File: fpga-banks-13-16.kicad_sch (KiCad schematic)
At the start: 48 parts, among them U14 XC7A100T-FGG484, U15 Oscillator_100MHz_AMJMEFB

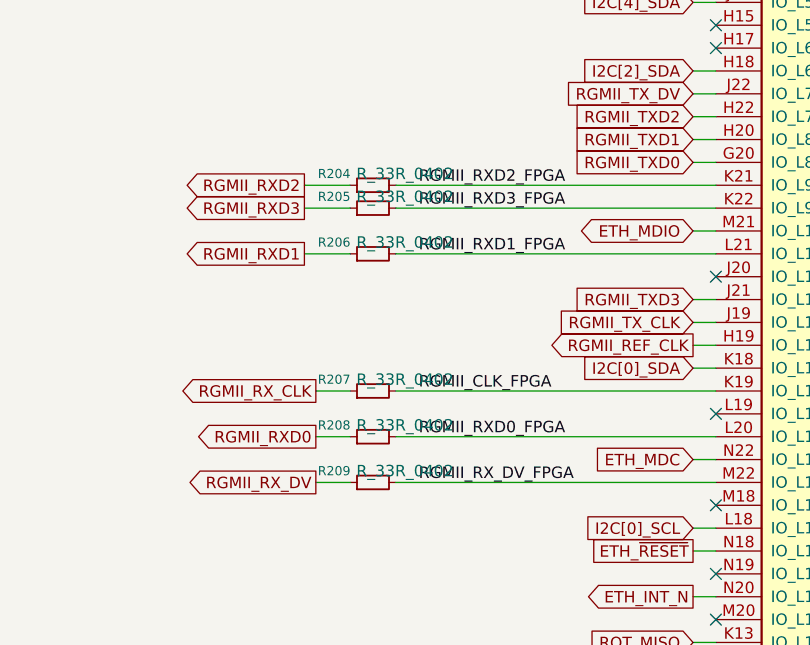
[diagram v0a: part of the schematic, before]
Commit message: version 1.0 complete
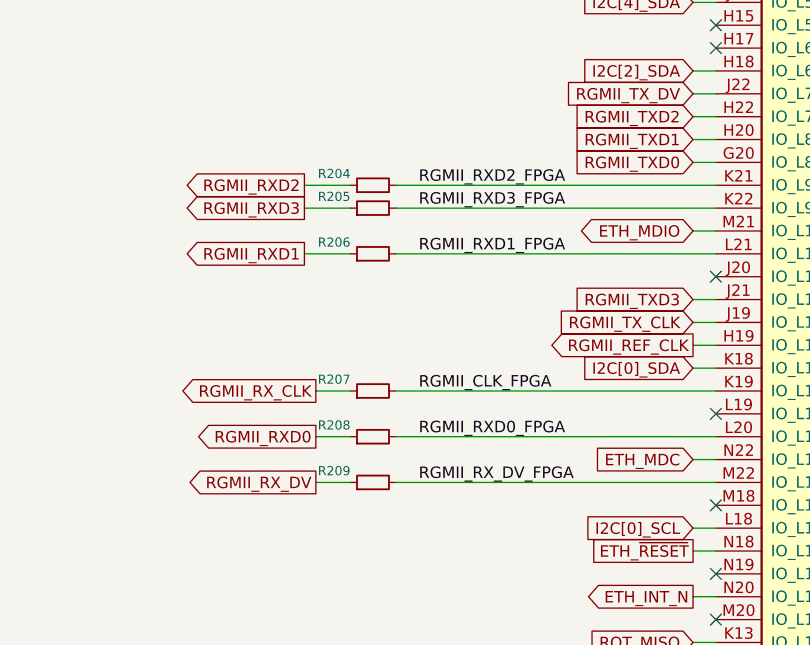
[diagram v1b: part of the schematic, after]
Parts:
- C92, C93, C94, C95: MPN C1210C476K8RACTU -> C1210C476K8RAC7210
- R133: MPN CR0402-FX-2201GLF -> AC0402FR-7D2K2L; Manufacturer Bourns -> YAGEO
- R134, R135: MPN CR0402-FX-4701GLF -> RC0402FR-7D4K7L; Manufacturer Bourns -> YAGEO
- R204, R205, R206, R207, R208, R209: MPN (none) -> MCS04020C3309FE000; Manufacturer (none) -> Vishay / Beyschlag
- U14: MPN XC7A100T-FGG484 -> XC7A100T-2FGG484C
- U15: MPN AMJMEFB-100.0000T -> ASEMB-100.000MHZ-XY-T

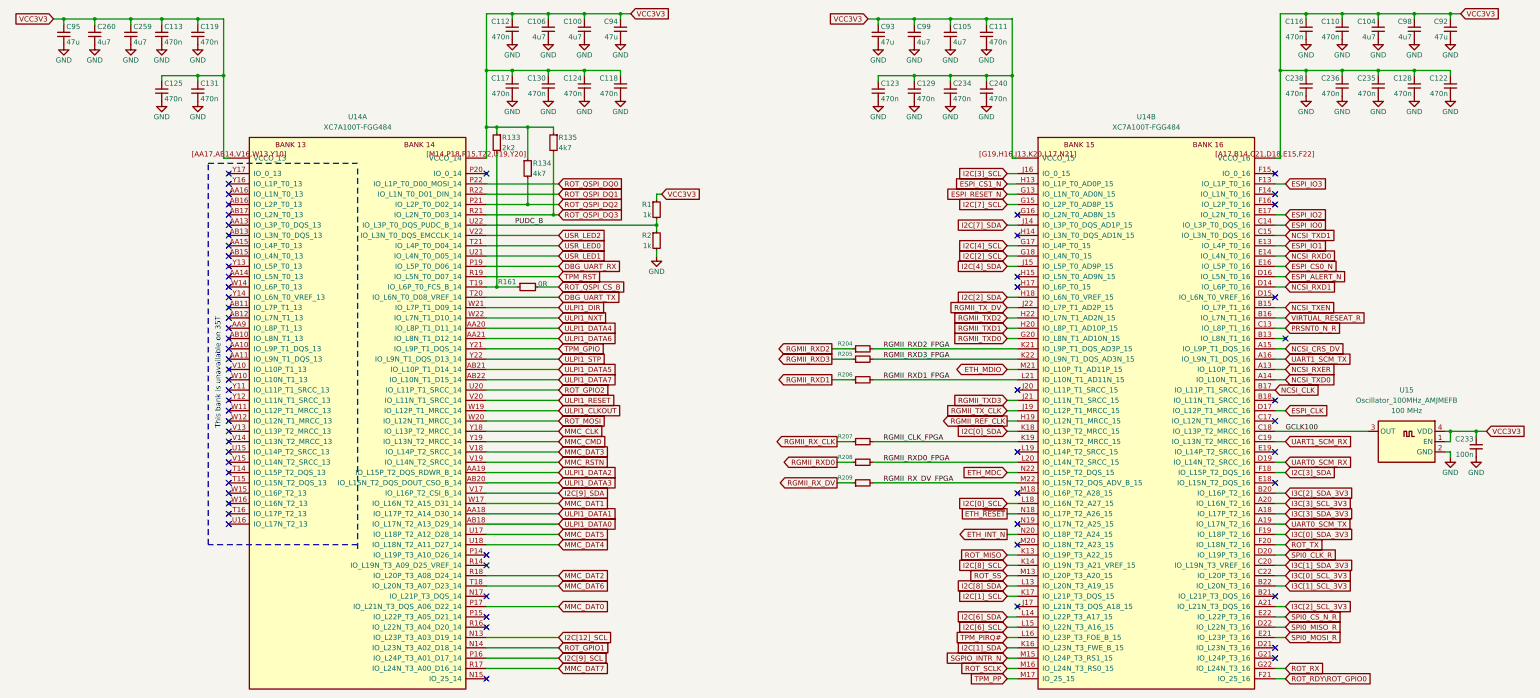
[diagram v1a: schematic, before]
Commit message: "In the process of upgrading the ddr memory"
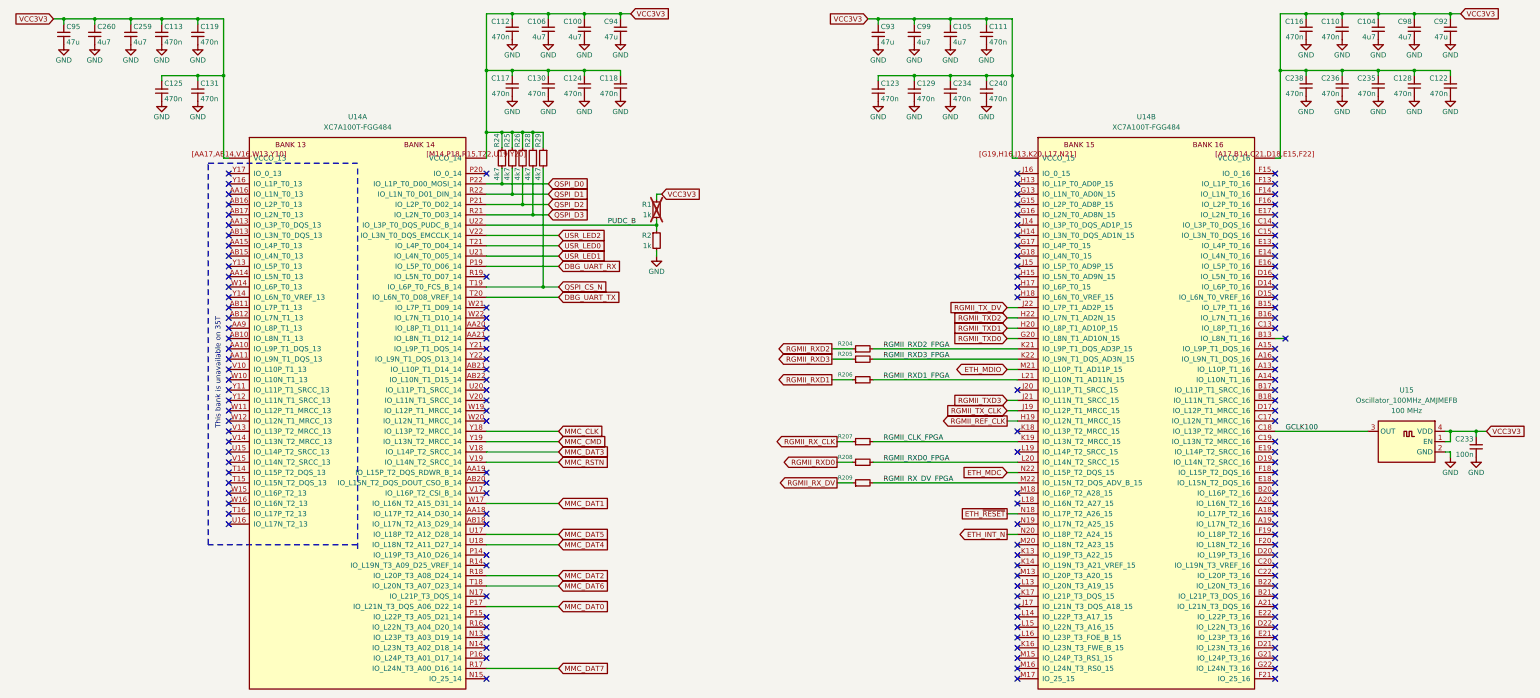
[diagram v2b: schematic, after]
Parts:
- removed R133: R_2k2_0402, antmicro-footprints:R_0402_1005Metric, symbol antmicroResistors0402:R_2k2_0402
- removed R134, R135: R_4k7_0402, antmicro-footprints:R_0402_1005Metric, symbol antmicroResistors0402:R_4k7_0402
- removed R161: R_0R_0402, antmicro-footprints:R_0402_1005Metric, symbol antmicroResistors0402:R_0R_0402
- added R24, R25, R26, R28, R29: R_4k7_0402, Resistor_SMD:R_0402_1005Metric, symbol antmicroResistors0402:R_4k7_0402
- C92, C93, C94, C95: footprint antmicro-footprints:C_1210_3225Metric -> Capacitor_SMD:C_1210_3225Metric
- R1: footprint antmicro-footprints:R_0402_1005Metric -> Resistor_SMD:R_0402_1005Metric; now not fitted; now left out of the parts list
- R2: footprint antmicro-footprints:R_0402_1005Metric -> Resistor_SMD:R_0402_1005Metric
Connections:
- net VCC3V3: now also R24.1, R25.1, R26.1, R28.1, R29.1
- net QSPI_CS_N: now reaches U14.T19 (IO_L6P_T0_FCS_B_14)
- net QSPI_CS_N: now also R29.2
- net ESPI_ALERT_N: no longer names the net of U14.D16 (IO_L5N_T0_16)
- net ESPI_CLK: no longer names the net of U14.D17 (IO_L12P_T1_MRCC_16)
- net ESPI_CS0_N: no longer names the net of U14.E16 (IO_L5P_T0_16)
- net ESPI_CS1_N: no longer names the net of U14.H13 (IO_L1P_T0_AD0P_15)
- net ESPI_IO0: no longer names the net of U14.C14 (IO_L3P_T0_DQS_16)
- net ESPI_IO1: no longer names the net of U14.E13 (IO_L4P_T0_16)
- net ESPI_IO2: no longer names the net of U14.E17 (IO_L2N_T0_16)
- net ESPI_IO3: no longer names the net of U14.F13 (IO_L1P_T0_16)
- net ESPI_RESET_N: no longer names the net of U14.G13 (IO_L1N_T0_AD0N_15)
- net I2C[0]_SCL: no longer names the net of U14.L18 (IO_L16N_T2_A27_15)
- net I2C[0]_SDA: no longer names the net of U14.K18 (IO_L13P_T2_MRCC_15)
- net I2C[12]_SCL: no longer names the net of U14.N13 (IO_L23P_T3_A03_D19_14)
- net I2C[1]_SCL: no longer names the net of U14.K17 (IO_L21P_T3_DQS_15)
- net I2C[1]_SDA: no longer names the net of U14.K16 (IO_L23N_T3_FWE_B_15)
- net I2C[2]_SCL: no longer names the net of U14.G18 (IO_L4N_T0_15)
- net I2C[2]_SDA: no longer names the net of U14.H18 (IO_L6N_T0_VREF_15)
- net I2C[3]_SCL: no longer names the net of U14.J16 (IO_0_15)
- net I2C[3]_SDA: no longer names the net of U14.F18 (IO_L15P_T2_DQS_16)
- net I2C[4]_SCL: no longer names the net of U14.G17 (IO_L4P_T0_15)
- net I2C[4]_SDA: no longer names the net of U14.J15 (IO_L5P_T0_AD9P_15)
- net I2C[6]_SCL: no longer names the net of U14.L15 (IO_L22N_T3_A16_15)
- net I2C[6]_SDA: no longer names the net of U14.L14 (IO_L22P_T3_A17_15)
- net I2C[7]_SCL: no longer names the net of U14.G15 (IO_L2P_T0_AD8P_15)
- net I2C[7]_SDA: no longer names the net of U14.J14 (IO_L3P_T0_DQS_AD1P_15)
- net I2C[8]_SCL: no longer names the net of U14.K14 (IO_L19N_T3_A21_VREF_15)
- net I2C[8]_SDA: no longer names the net of U14.L13 (IO_L20N_T3_A19_15)
- net I2C[9]_SCL: no longer names the net of U14.P16 (IO_L24P_T3_A01_D17_14)
- net I2C[9]_SDA: no longer names the net of U14.V17 (IO_L16P_T2_CSI_B_14)
- net I3C[0]_SCL_3V3: no longer names the net of U14.C22 (IO_L20P_T3_16)
- net I3C[0]_SDA_3V3: no longer names the net of U14.F19 (IO_L18P_T2_16)
- net I3C[1]_SCL_3V3: no longer names the net of U14.B22 (IO_L20N_T3_16)
- net I3C[1]_SDA_3V3: no longer names the net of U14.C20 (IO_L19N_T3_VREF_16)
- net I3C[2]_SCL_3V3: no longer names the net of U14.A21 (IO_L21N_T3_DQS_16)
- net I3C[2]_SDA_3V3: no longer names the net of U14.B20 (IO_L16P_T2_16)
- net I3C[3]_SCL_3V3: no longer names the net of U14.A20 (IO_L16N_T2_16)
- net I3C[3]_SDA_3V3: no longer names the net of U14.A18 (IO_L17P_T2_16)
- net NCSI_CLK: no longer names the net of U14.B17 (IO_L11P_T1_SRCC_16)
- net NCSI_CRS_DV: no longer names the net of U14.A15 (IO_L9P_T1_DQS_16)
- net NCSI_RXD0: no longer names the net of U14.E14 (IO_L4N_T0_16)
- net NCSI_RXD1: no longer names the net of U14.D14 (IO_L6P_T0_16)
- net NCSI_RXER: no longer names the net of U14.A13 (IO_L10P_T1_16)
- net NCSI_TXD0: no longer names the net of U14.A14 (IO_L10N_T1_16)
- net NCSI_TXD1: no longer names the net of U14.C15 (IO_L3N_T0_DQS_16)
- net NCSI_TXEN: no longer names the net of U14.B15 (IO_L7P_T1_16)
- net PRSNT0_N_R: no longer names the net of U14.C13 (IO_L8P_T1_16)
- net ROT_GPIO1: no longer names the net of U14.N14 (IO_L23N_T3_A02_D18_14)
- net ROT_GPIO2: no longer names the net of U14.U20 (IO_L11P_T1_SRCC_14)
- net ROT_MISO: no longer names the net of U14.K13 (IO_L19P_T3_A22_15)
- net ROT_MOSI: no longer names the net of U14.W20 (IO_L12N_T1_MRCC_14)
- net ROT_QSPI_DQ0 renamed QSPI_D0
- net QSPI_D0: now also R24.2
- net ROT_QSPI_DQ1 renamed QSPI_D1
- net QSPI_D1: now also R25.2
- net ROT_QSPI_DQ2 renamed QSPI_D2
- net QSPI_D2: now also R26.2
- net ROT_QSPI_DQ3 renamed QSPI_D3
- net QSPI_D3: now also R28.2
- net ROT_RDY\ROT_GPIO0: no longer names the net of U14.F21 (IO_25_16)
- net ROT_RX: no longer names the net of U14.G22 (IO_L24N_T3_16)
- net ROT_SCLK: no longer names the net of U14.M16 (IO_L24N_T3_RS0_15)
- net ROT_SS: no longer names the net of U14.M13 (IO_L20P_T3_A20_15)
- net ROT_TX: no longer names the net of U14.F20 (IO_L18N_T2_16)
- net SGPIO_INTR_N: no longer names the net of U14.M15 (IO_L24P_T3_RS1_15)
- net SPI0_CLK_R: no longer names the net of U14.D20 (IO_L19P_T3_16)
- net SPI0_CS_N_R: no longer names the net of U14.E22 (IO_L22P_T3_16)
- net SPI0_MISO_R: no longer names the net of U14.D22 (IO_L22N_T3_16)
- net SPI0_MOSI_R: no longer names the net of U14.E21 (IO_L23P_T3_16)
- net TPM_GPIO: no longer names the net of U14.Y21 (IO_L9P_T1_DQS_14)
- net TPM_PIRQ#: no longer names the net of U14.L16 (IO_L23P_T3_FOE_B_15)
- net TPM_PP: no longer names the net of U14.M17 (IO_25_15)
- net TPM_RST: no longer names the net of U14.R19 (IO_L5N_T0_D07_14)
- net UART0_SCM_RX: no longer names the net of U14.D19 (IO_L14N_T2_SRCC_16)
- net UART0_SCM_TX: no longer names the net of U14.A19 (IO_L17N_T2_16)
- net UART1_SCM_RX: no longer names the net of U14.C19 (IO_L13N_T2_MRCC_16)
- net UART1_SCM_TX: no longer names the net of U14.A16 (IO_L9N_T1_DQS_16)
- net ULPI1_CLKOUT: no longer names the net of U14.W19 (IO_L12P_T1_MRCC_14)
- net ULPI1_DATA0: no longer names the net of U14.AB18 (IO_L17N_T2_A13_D29_14)
- net ULPI1_DATA1: no longer names the net of U14.AA18 (IO_L17P_T2_A14_D30_14)
- net ULPI1_DATA2: no longer names the net of U14.AA19 (IO_L15P_T2_DQS_RDWR_B_14)
- net ULPI1_DATA3: no longer names the net of U14.AB20 (IO_L15N_T2_DQS_DOUT_CSO_B_14)
- net ULPI1_DATA4: no longer names the net of U14.AA20 (IO_L8P_T1_D11_14)
- net ULPI1_DATA5: no longer names the net of U14.AB21 (IO_L10P_T1_D14_14)
- net ULPI1_DATA6: no longer names the net of U14.AA21 (IO_L8N_T1_D12_14)
- net ULPI1_DATA7: no longer names the net of U14.AB22 (IO_L10N_T1_D15_14)
- net ULPI1_DIR: no longer names the net of U14.W21 (IO_L7P_T1_D09_14)
- net ULPI1_NXT: no longer names the net of U14.W22 (IO_L7N_T1_D10_14)
- net ULPI1_RESET: no longer names the net of U14.V20 (IO_L11N_T1_SRCC_14)
- net ULPI1_STP: no longer names the net of U14.Y22 (IO_L9N_T1_DQS_D13_14)
- net VIRTUAL_RESEAT_R: no longer names the net of U14.B16 (IO_L7N_T1_16)
- no-connect marks 64 -> 145
